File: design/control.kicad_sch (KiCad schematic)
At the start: 30 parts, among them J1 BNC, J10 Conn_01x03_Pin, J2 BWSMA-KWE-Z001, J3 BWSMA-KE-Z001, J4 BWSMA-KE-Z001, J5 SHOU HAN TYPE-C 14P CC-2.6, J6 Conn_01x03_Pin, J9 Conn_01x04_Pin, U1 STM32F303RETx, U2 USBLC6-2SC6, U3 FT230XQ

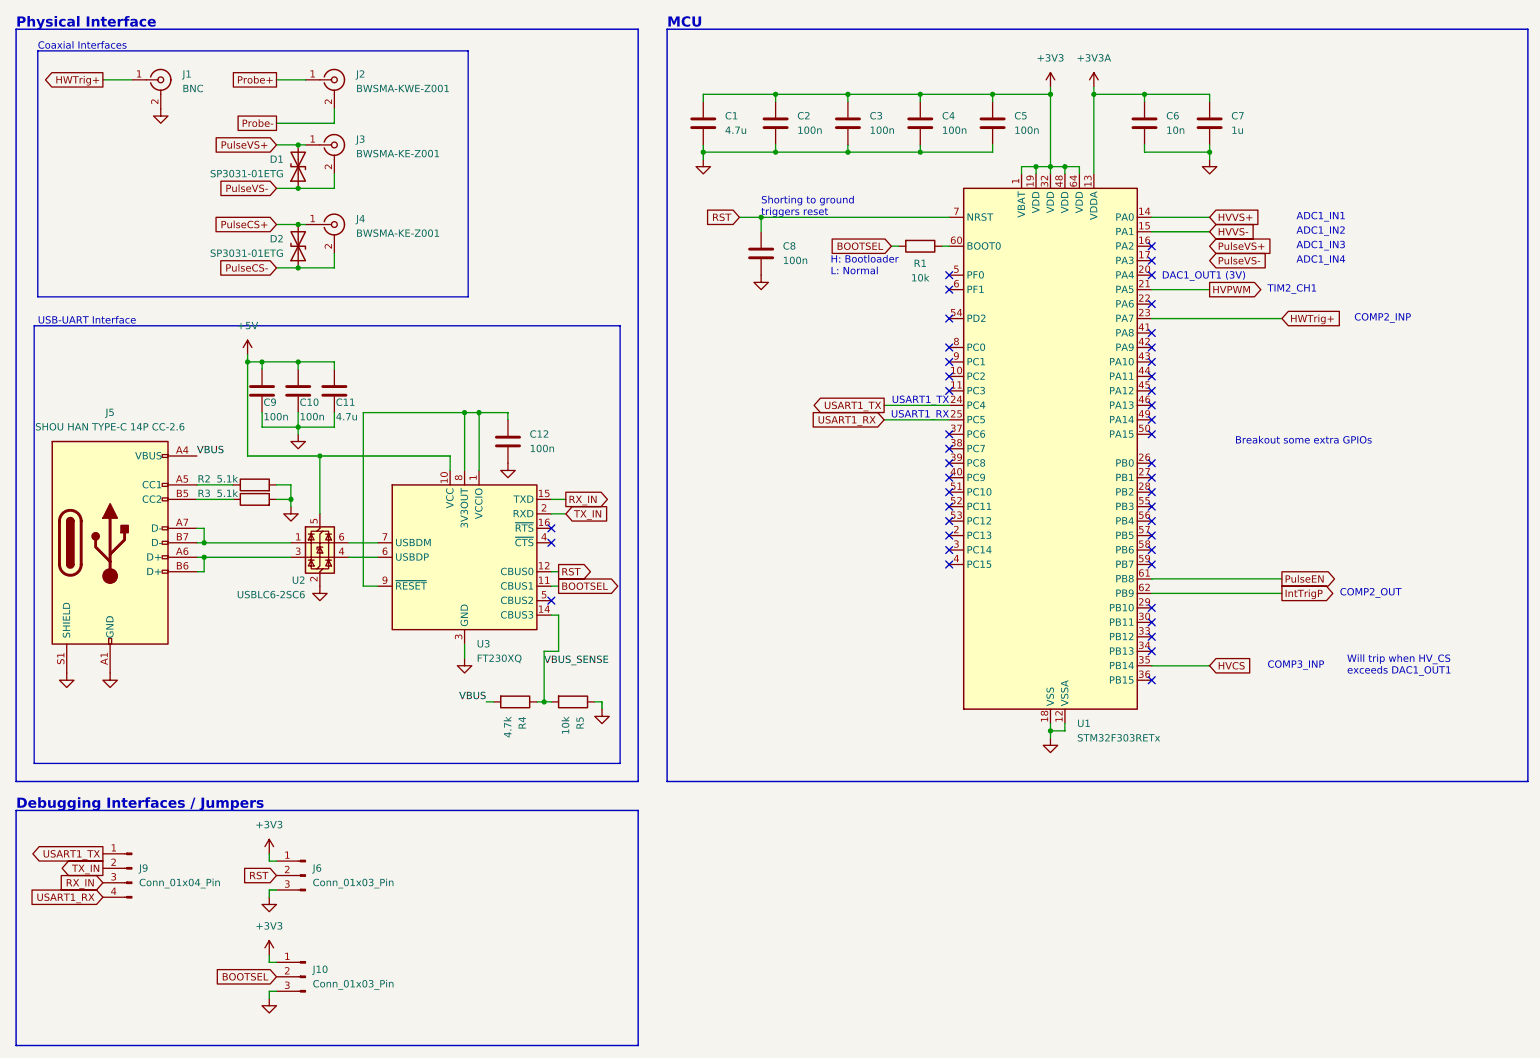
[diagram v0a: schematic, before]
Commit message: Cleanup
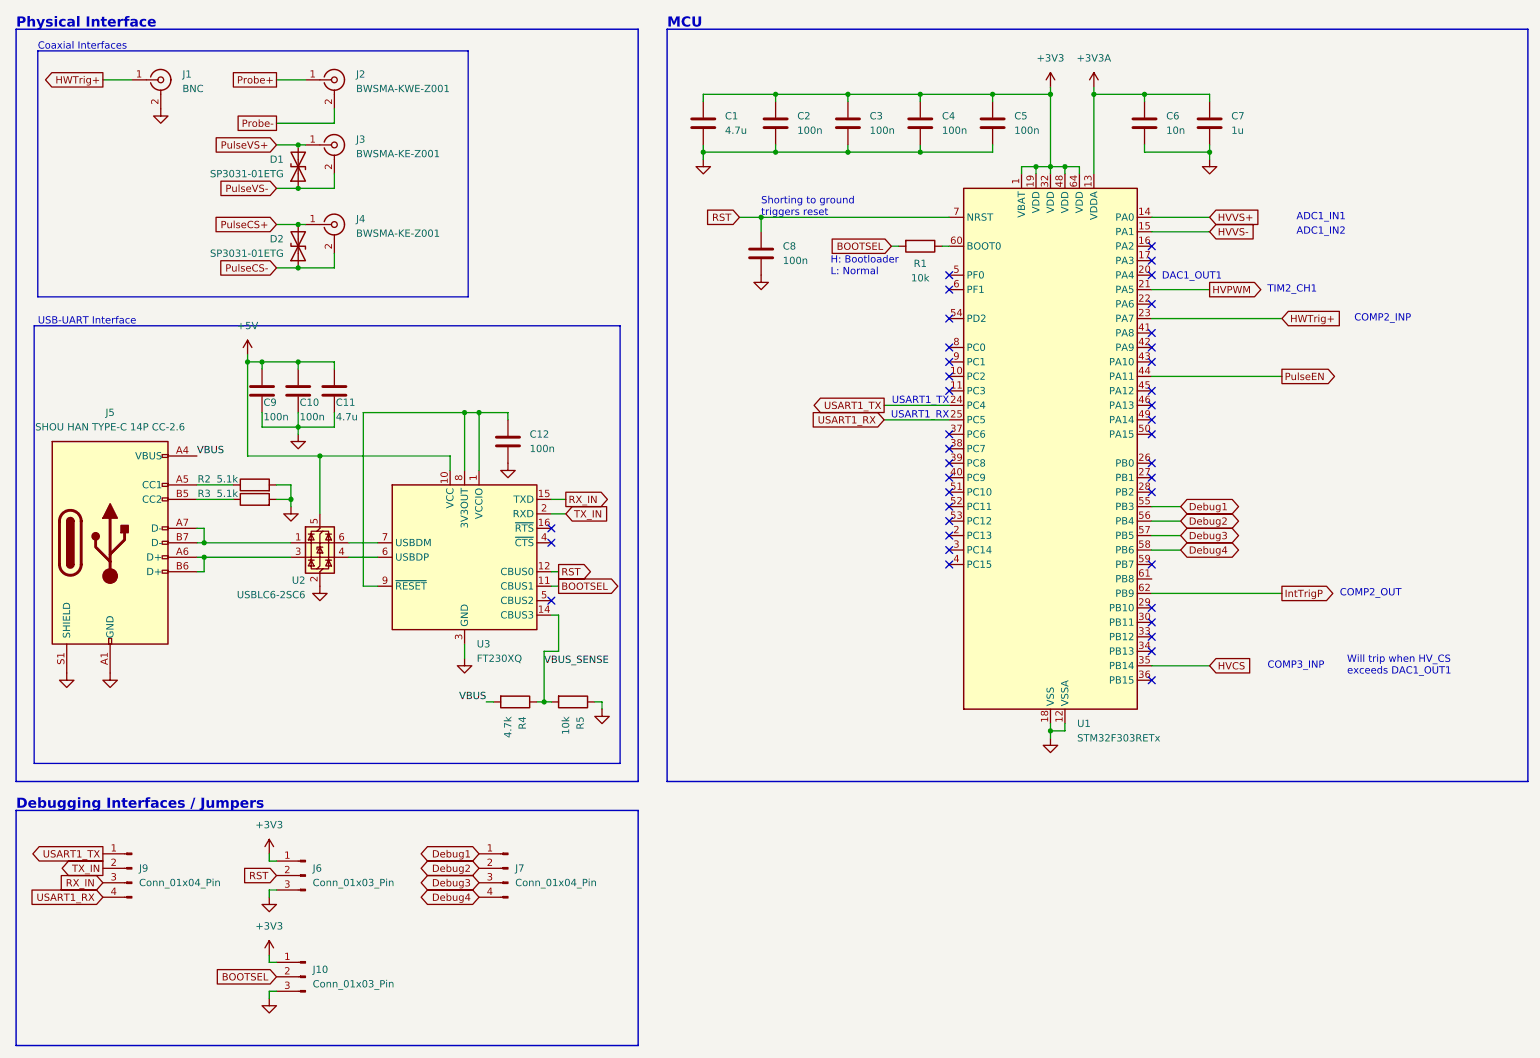
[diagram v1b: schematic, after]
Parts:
- added J7: Conn_01x04_Pin, Connector_PinHeader_2.54mm:PinHeader_1x04_P2.54mm_Vertical, symbol Connector:Conn_01x04_Pin
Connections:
- net PulseEN: now also U1.44 (PA11); no longer U1.61 (PB8)
- net Debug1: now reaches U1.55 (PB3)
- net Debug1: now also J7.1 (Pin_1)
- net Debug2: now reaches U1.56 (PB4)
- net Debug2: now also J7.2 (Pin_2)
- net Debug3: now reaches U1.57 (PB5)
- net Debug3: now also J7.3 (Pin_3)
- net Debug4: now reaches U1.58 (PB6)
- net Debug4: now also J7.4 (Pin_4)
- no-connect marks 45 -> 40
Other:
- note added: "DAC1_OUT1"
- note removed: "ADC1_IN3"
- note removed: "ADC1_IN4"
- note removed: "Breakout some extra GPIOs"
- note removed: "DAC1_OUT1 (3V)"
